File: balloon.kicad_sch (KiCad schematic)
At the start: 13 parts, among them SW1 SW_Push, U1 STM32L431RBTx, Y1 Crystal

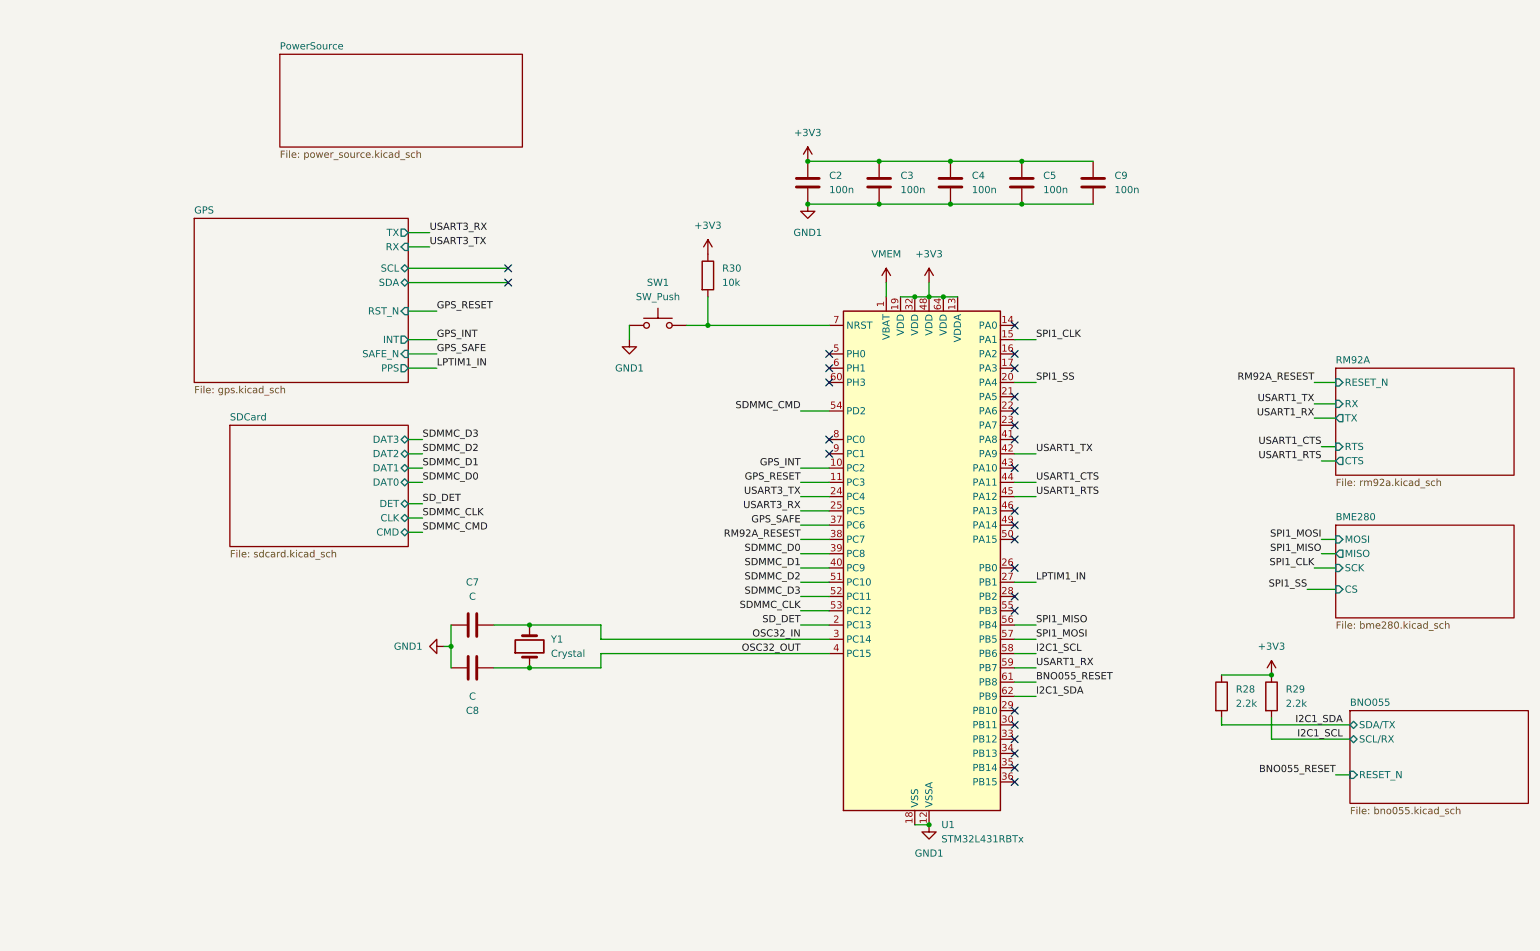
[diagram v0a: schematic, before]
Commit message: make board
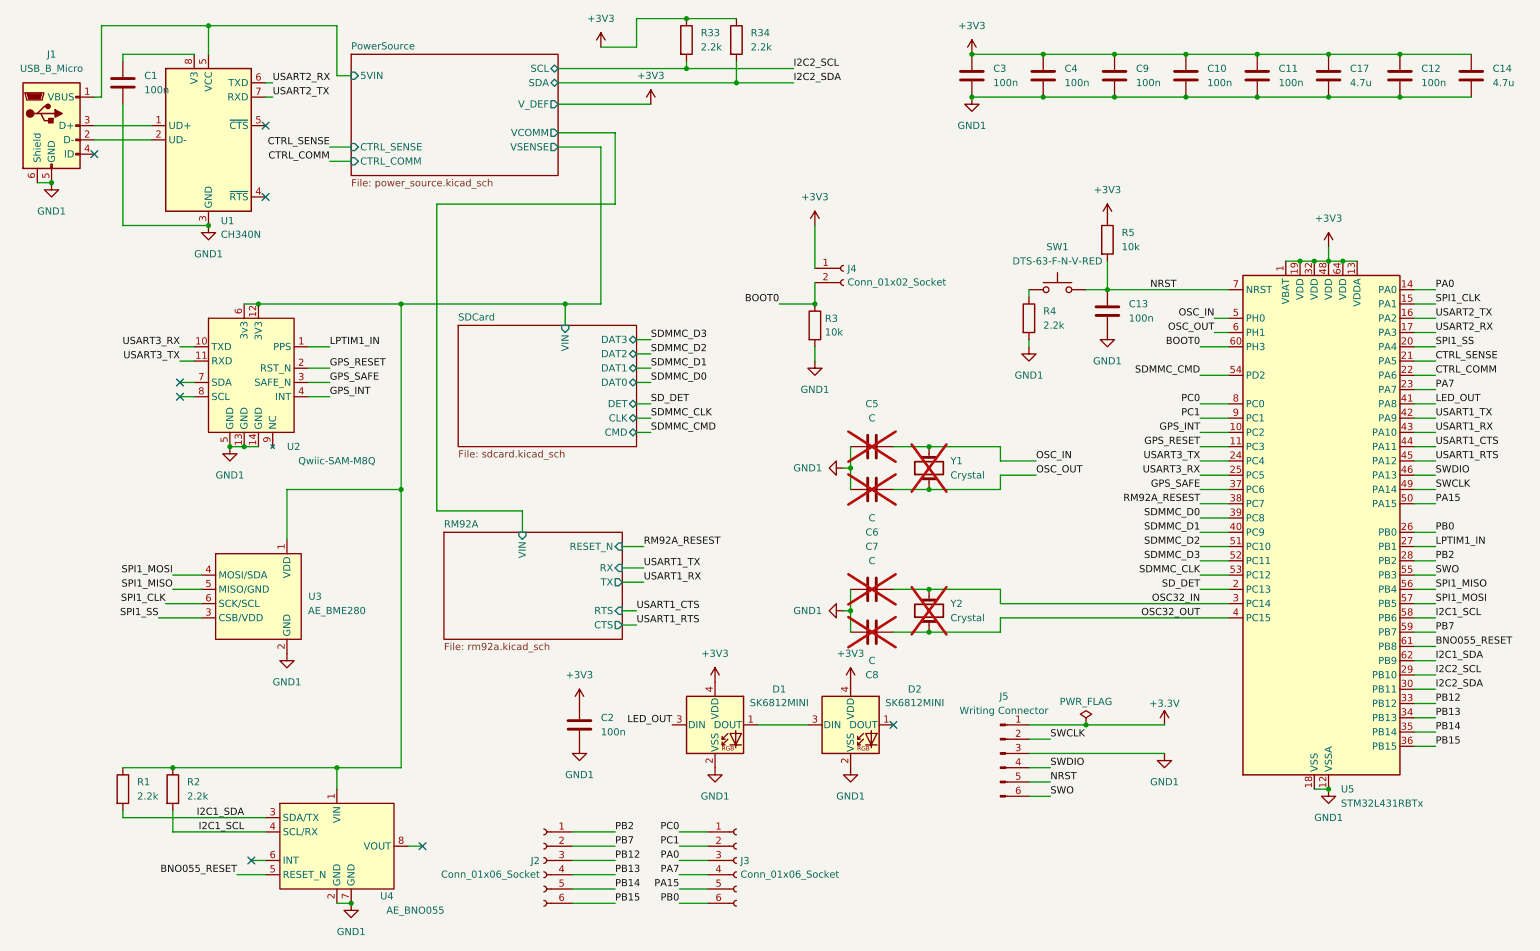
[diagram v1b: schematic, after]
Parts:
- added C1, C12, C13, C2: 100n, Capacitor_SMD:C_0603_1608Metric_Pad1.08x0.95mm_HandSolder, symbol Device:C
- added C14, C17: 4.7u, Capacitor_SMD:C_0603_1608Metric_Pad1.08x0.95mm_HandSolder, symbol Device:C
- added C5, C6: C, Capacitor_SMD:C_0603_1608Metric_Pad1.08x0.95mm_HandSolder, symbol Device:C
- added D1, D2: SK6812MINI, LED_SMD:LED_SK6812MINI_PLCC4_3.5x3.5mm_P1.75mm, symbol LED:SK6812MINI
- added J1: USB_B_Micro, Connector_USB:USB_Micro-B_Molex_47346-0001, symbol Connector:USB_B_Micro
- added J2, J3: Conn_01x06_Socket, Connector_PinHeader_2.54mm:PinHeader_1x06_P2.54mm_Vertical, symbol Connector:Conn_01x06_Socket
- added J4: Conn_01x02_Socket, Connector_PinHeader_2.54mm:PinHeader_1x02_P2.54mm_Vertical, symbol Connector:Conn_01x02_Socket
- added J5: Writing Connector, Connector_PinSocket_2.54mm:PinSocket_1x06_P2.54mm_Vertical, symbol Connector:Conn_01x06_Pin
- added R3: 10k, Resistor_SMD:R_0603_1608Metric_Pad0.98x0.95mm_HandSolder, symbol Device:R
- added R33, R34, R4: 2.2k, Resistor_SMD:R_0603_1608Metric_Pad0.98x0.95mm_HandSolder, symbol Device:R
- added U1: CH340N, Package_SO:MSOP-10_3x3mm_P0.5mm, symbol balloon_lib:CH340N
- added U2: Qwiic-SAM-M8Q, balloon:Qwiic_SAM-M8Q, symbol balloon_lib:Qwiic-SAM-M8Q
- added U3: AE_BME280, balloon:AE_BNE280, symbol balloon_lib:BME280
- added U4: AE_BNO055, balloon:AE-BNO055, symbol balloon_lib:BNO055
- added Y1: Crystal, Crystal:Crystal_C38-LF_D3.0mm_L8.0mm_Vertical, symbol Device:Crystal
- C10: renamed from C5; footprint (none) -> Capacitor_SMD:C_0603_1608Metric_Pad1.08x0.95mm_HandSolder
- C11: renamed from C9; footprint (none) -> Capacitor_SMD:C_0603_1608Metric_Pad1.08x0.95mm_HandSolder
- C3: renamed from C2; footprint (none) -> Capacitor_SMD:C_0603_1608Metric_Pad1.08x0.95mm_HandSolder
- C4: renamed from C3; footprint (none) -> Capacitor_SMD:C_0603_1608Metric_Pad1.08x0.95mm_HandSolder
- C7, C8: footprint (none) -> Capacitor_SMD:C_0603_1608Metric_Pad1.08x0.95mm_HandSolder; now not fitted
- C9: renamed from C4; footprint (none) -> Capacitor_SMD:C_0603_1608Metric_Pad1.08x0.95mm_HandSolder
- R1: renamed from R28; footprint (none) -> Resistor_SMD:R_0603_1608Metric_Pad0.98x0.95mm_HandSolder
- R2: renamed from R29; footprint (none) -> Resistor_SMD:R_0603_1608Metric_Pad0.98x0.95mm_HandSolder
- R5: renamed from R30; footprint (none) -> Resistor_SMD:R_0603_1608Metric_Pad0.98x0.95mm_HandSolder
- SW1: value SW_Push -> DTS-63-F-N-V-RED; footprint (none) -> Button_Switch_THT:SW_PUSH_6mm
- Y2: renamed from Y1; footprint (none) -> Crystal:Crystal_C38-LF_D3.0mm_L8.0mm_Vertical; now not fitted
- renumbered U1 to U5
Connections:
- net VMEM is gone; now on net +3V3: U5.1 (VBAT)
- net +3V3: now also C12.1, C14.1, C17.1, C2.1, D1.4 (VDD), D2.4 (VDD), J4.1 (Pin_1), R33.1, R34.1; no longer R1.1, R2.1
- net BNO055_RESET: now also U4.5 (RESET_N)
- net GND1: now also C1.2, C12.2, C13.2, C14.2, C17.2, C2.2, C5.1, C6.2, D1.2 (VSS), D2.2 (VSS), J1.5 (GND), J1.6 (Shield), J5.3 (Pin_3), R3.2, R4.2, U1.3 (GND), U2.13 (GND), U2.14 (GND), U2.5 (GND), U3.2 (GND), U4.2 (GND), U4.7 (GND); no longer SW1.1
- net GPS_INT: now also U2.4 (INT)
- net GPS_RESET: now also U2.2 (RST_N)
- net GPS_SAFE: now also U2.3 (SAFE_N)
- net I2C1_SCL: now also U4.4 (SCL/RX)
- net I2C1_SDA: now also U4.3 (SDA/TX)
- net LPTIM1_IN: now also U2.1 (PPS)
- net SPI1_CLK: now also U3.6 (SCK/SCL)
- net SPI1_MISO: now also U3.5 (MISO/GND)
- net SPI1_MOSI: now also U3.4 (MOSI/SDA)
- net SPI1_SS: now also U3.3 (CSB/VDD)
- net USART1_RX: now also U5.43 (PA10); no longer U5.59 (PB7)
- net USART3_RX: now also U2.10 (TXD)
- net USART3_TX: now also U2.11 (RXD)
- net NRST: now reaches R5.2, SW1.2, U5.7 (NRST)
- net NRST: now also C13.1, J5.5 (Pin_5)
- net PA0: now reaches U5.14 (PA0)
- net PA0: now also J3.3 (Pin_3)
- net USART2_TX: now reaches U5.16 (PA2)
- net USART2_TX: now also U1.7 (RXD)
- net USART2_RX: now reaches U5.17 (PA3)
- net USART2_RX: now also U1.6 (TXD)
- net CTRL_SENSE: now reaches U5.21 (PA5)
- net CTRL_COMM: now reaches U5.22 (PA6)
- net PA7: now reaches U5.23 (PA7)
- net PA7: now also J3.4 (Pin_4)
- net PB0: now reaches U5.26 (PB0)
- net PB0: now also J3.6 (Pin_6)
- net PB2: now reaches U5.28 (PB2)
- net PB2: now also J2.1 (Pin_1)
- net I2C2_SCL: now reaches U5.29 (PB10)
- net I2C2_SCL: now also R33.2
- net I2C2_SDA: now reaches U5.30 (PB11)
- net I2C2_SDA: now also R34.2
- net PB12: now reaches U5.33 (PB12)
- net PB12: now also J2.3 (Pin_3)
- net PB13: now reaches U5.34 (PB13)
- net PB13: now also J2.4 (Pin_4)
- net PB14: now reaches U5.35 (PB14)
- net PB14: now also J2.5 (Pin_5)
- net PB15: now reaches U5.36 (PB15)
- net PB15: now also J2.6 (Pin_6)
- net LED_OUT: now reaches U5.41 (PA8)
- net LED_OUT: now also D1.3 (DIN)
- net SWDIO: now reaches U5.46 (PA13)
- net SWDIO: now also J5.4 (Pin_4)
- net SWCLK: now reaches U5.49 (PA14)
- net SWCLK: now also J5.2 (Pin_2)
- net OSC_IN: now reaches U5.5 (PH0)
- net OSC_IN: now also C5.2, Y1.2
- net PA15: now reaches U5.50 (PA15)
- net PA15: now also J3.5 (Pin_5)
- net SWO: now reaches U5.55 (PB3)
- net SWO: now also J5.6 (Pin_6)
- net OSC_OUT: now reaches U5.6 (PH1)
- net OSC_OUT: now also C6.1, Y1.1
- net BOOT0: now reaches U5.60 (PH3)
- net BOOT0: now also J4.2 (Pin_2), R3.1
- net PC0: now reaches U5.8 (PC0)
- net PC0: now also J3.1 (Pin_1)
- net PC1: now reaches U5.9 (PC1)
- net PC1: now also J3.2 (Pin_2)
- new net: J1.2 (D-), U1.2 (UD-)
- new net: J1.3 (D+), U1.1 (UD+)
- new net: R4.1, SW1.1
- new net: C1.1, U1.8 (V3)
- new net: D1.1 (DOUT), D2.3 (DIN)
- new net +3.3V: J5.1 (Pin_1)
- new net PB7: J2.2 (Pin_2), U5.59 (PB7)
- new net PowerSource/5VIN: J1.1 (VBUS), U1.5 (~{CTS})
- new net PowerSource/VSENSE: R1.1, R2.1, U2.12 (3V3), U2.6 (3v3), U3.1 (VDD), U4.1 (VIN)
- no-connect marks 27 -> 8
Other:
- removed sheet BME280
- removed sheet BNO055
- removed sheet GPS
- sheet PowerSource ports: added 5VIN, CTRL_COMM, CTRL_SENSE, SCL, SDA, VCOMM, VSENSE, V_DEF; removed none
- sheet RM92A ports: added VIN; removed none
- sheet SDCard ports: added VIN; removed none
- moved on the sheet: C10, C11, C3, C4, C9, R1, R2, R5, SW1, U5
